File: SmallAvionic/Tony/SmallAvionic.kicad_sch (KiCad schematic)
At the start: 0 parts

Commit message: 完成基本開機電路
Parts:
- added C1, C2, C3, C4, C6, C9: 100n, symbol Device:C
- added C5, C7: 10u, symbol Device:C
- added C8: 1n, symbol Device:C
- added FB1: FerriteBead 120R @ 100M, symbol Device:FerriteBead
- added J1: Conn_01x02_Pin, symbol Connector:Conn_01x02_Pin
- added R1, R2: 10k, symbol Device:R
- added SW1: SW_Push, symbol Switch:SW_Push
- added TP1: TestPoint, symbol Connector:TestPoint
- added U1: STM32F103C8Tx, Package_QFP:LQFP-48_7x7mm_P0.5mm, symbol MCU_ST_STM32F1:STM32F103C8Tx
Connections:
- new net: C8.1, FB1.2
- new net: C9.1, SW1.2, U1.7 (NRST)
- new net: R1.1, TP1.1, U1.44 (BOOT0)
- new net: R2.1, U1.20 (PB2)
- new net +3.3V: C1.1, C2.1, C3.1, C4.1, C5.1, U1.1 (VBAT), U1.24 (VDD), U1.36 (VDD), U1.48 (VDD)
- new net +3.3VA: C6.1, C7.1, FB1.1, U1.9 (VDDA)
- new net GND: C1.2, C2.2, C3.2, C4.2, C5.2, C6.2, C7.2, C8.2, C9.2, R1.2, R2.2, SW1.1, U1.23 (VSS), U1.35 (VSS), U1.47 (VSS), U1.8 (VSSA)

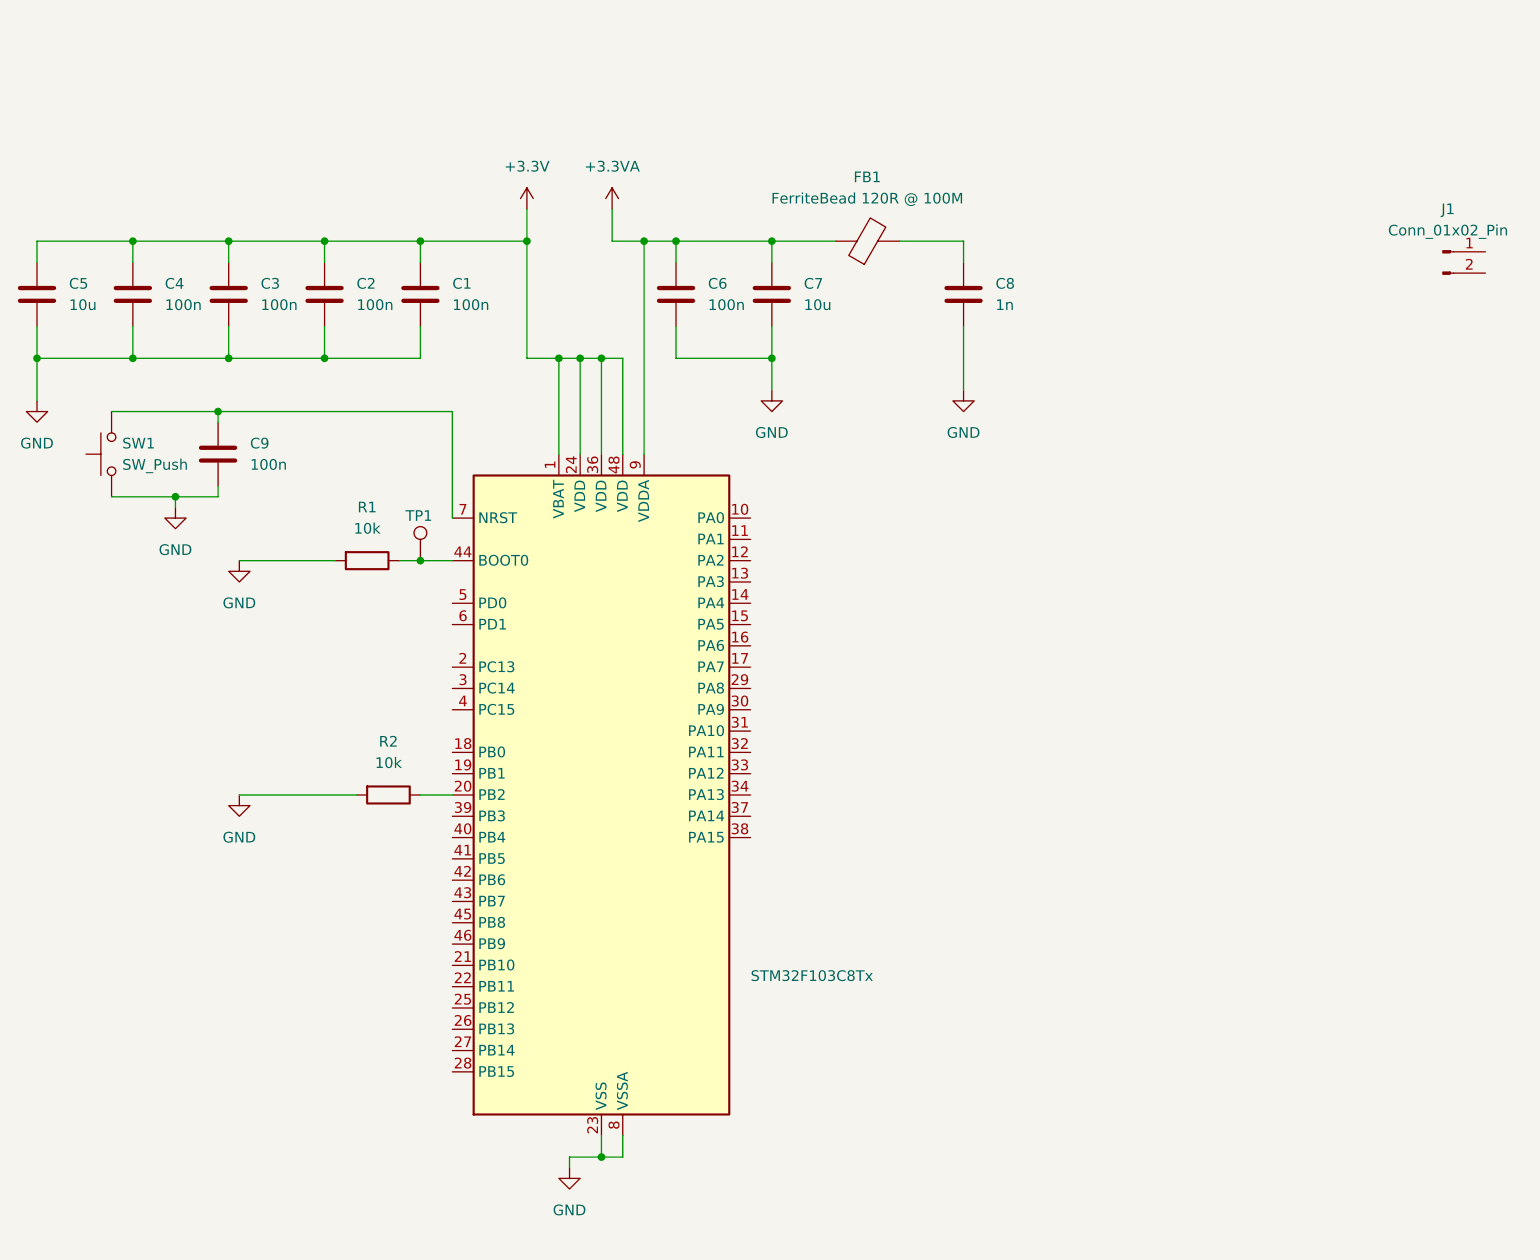
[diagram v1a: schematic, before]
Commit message: 進度到usb
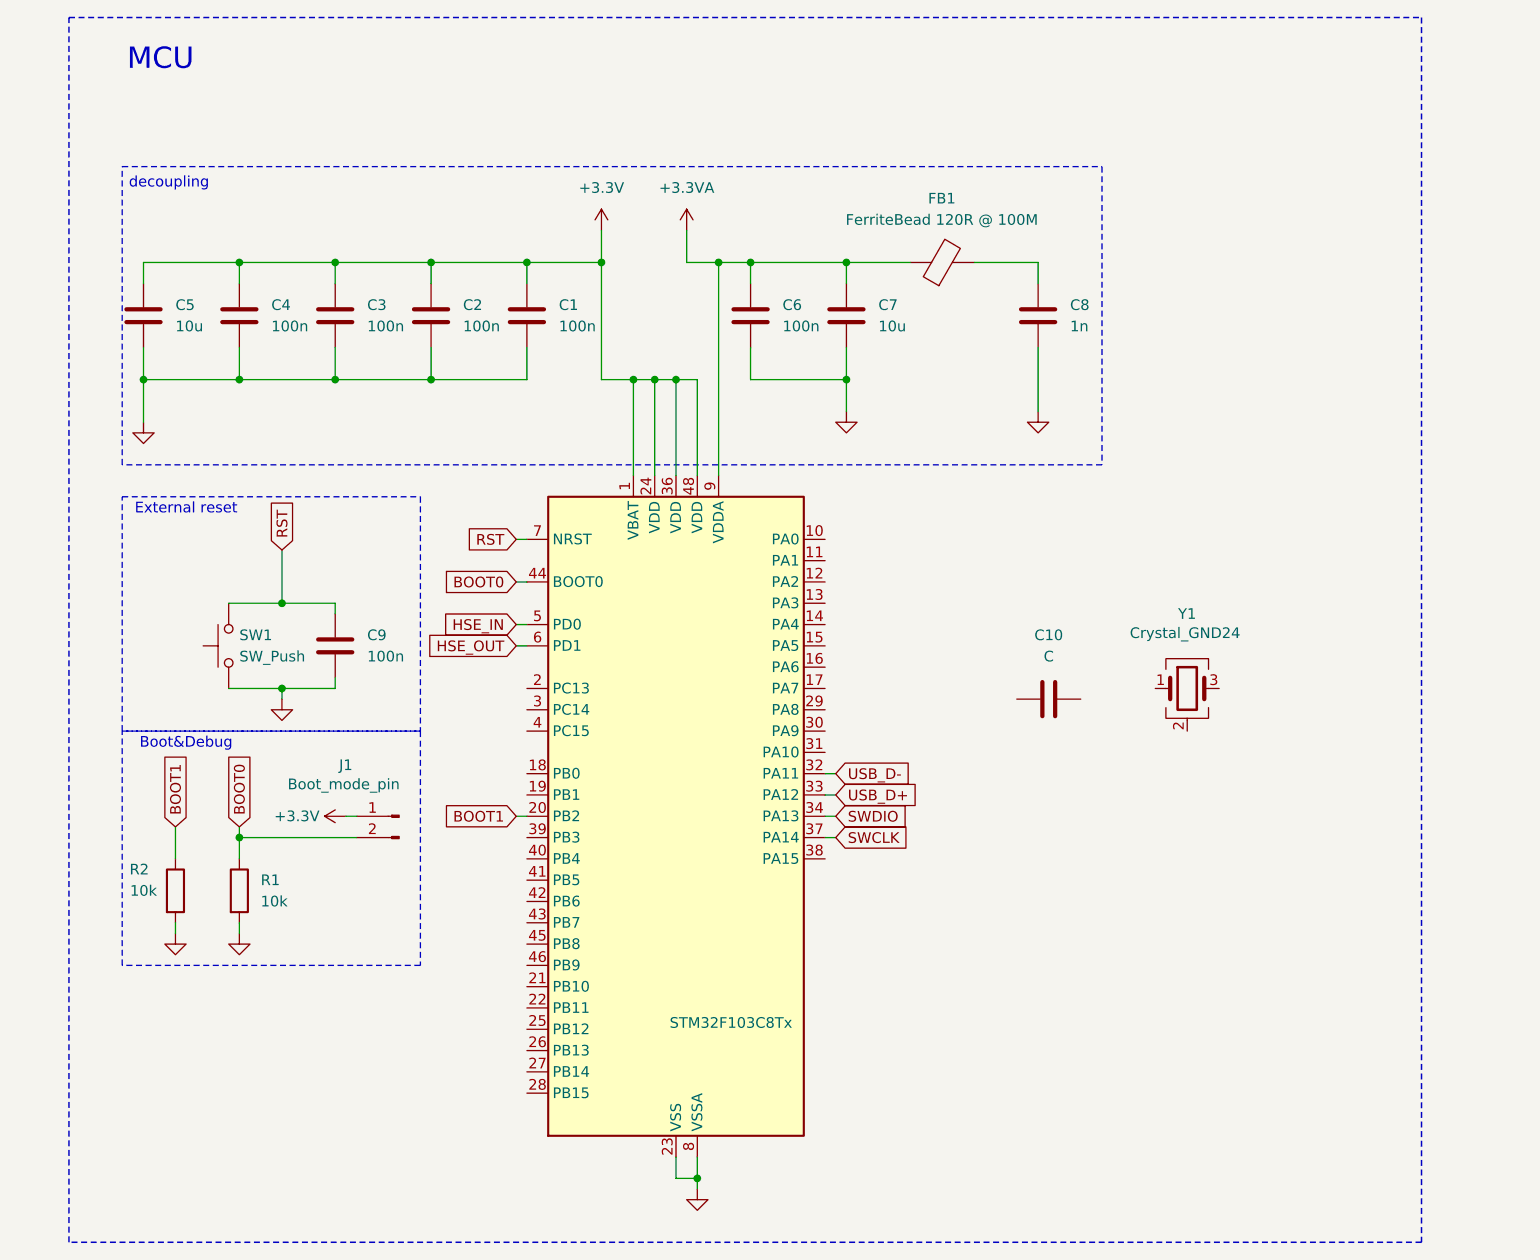
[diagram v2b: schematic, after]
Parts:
- removed TP1: TestPoint, symbol Connector:TestPoint
- added C10: C, symbol Device:C
- added Y1: Crystal_GND24, symbol Device:Crystal_GND24
- J1: value Conn_01x02_Pin -> Boot_mode_pin
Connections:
- net +3.3V: now also J1.1 (Pin_1)
- net RST: now reaches C9.1, SW1.2, U1.7 (NRST)
- net BOOT0: now reaches R1.1, U1.44 (BOOT0)
- net BOOT0: now also J1.2 (Pin_2)
- net BOOT1: now reaches R2.1, U1.20 (PB2)
- net USB_D-: now reaches U1.32 (PA11)
- net USB_D+: now reaches U1.33 (PA12)
- net SWDIO: now reaches U1.34 (PA13)
- net SWCLK: now reaches U1.37 (PA14)
- net HSE_IN: now reaches U1.5 (PD0)
- net HSE_OUT: now reaches U1.6 (PD1)
- new net: Y1.2 (G), Y1.4 (G)
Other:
- note added: "Boot&Debug"
- note added: "External reset"
- note added: "MCU"
- note added: "decoupling"
- moved on the sheet: C1, C2, C3, C4, C5, C6, C7, C8, C9, FB1, J1, R1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

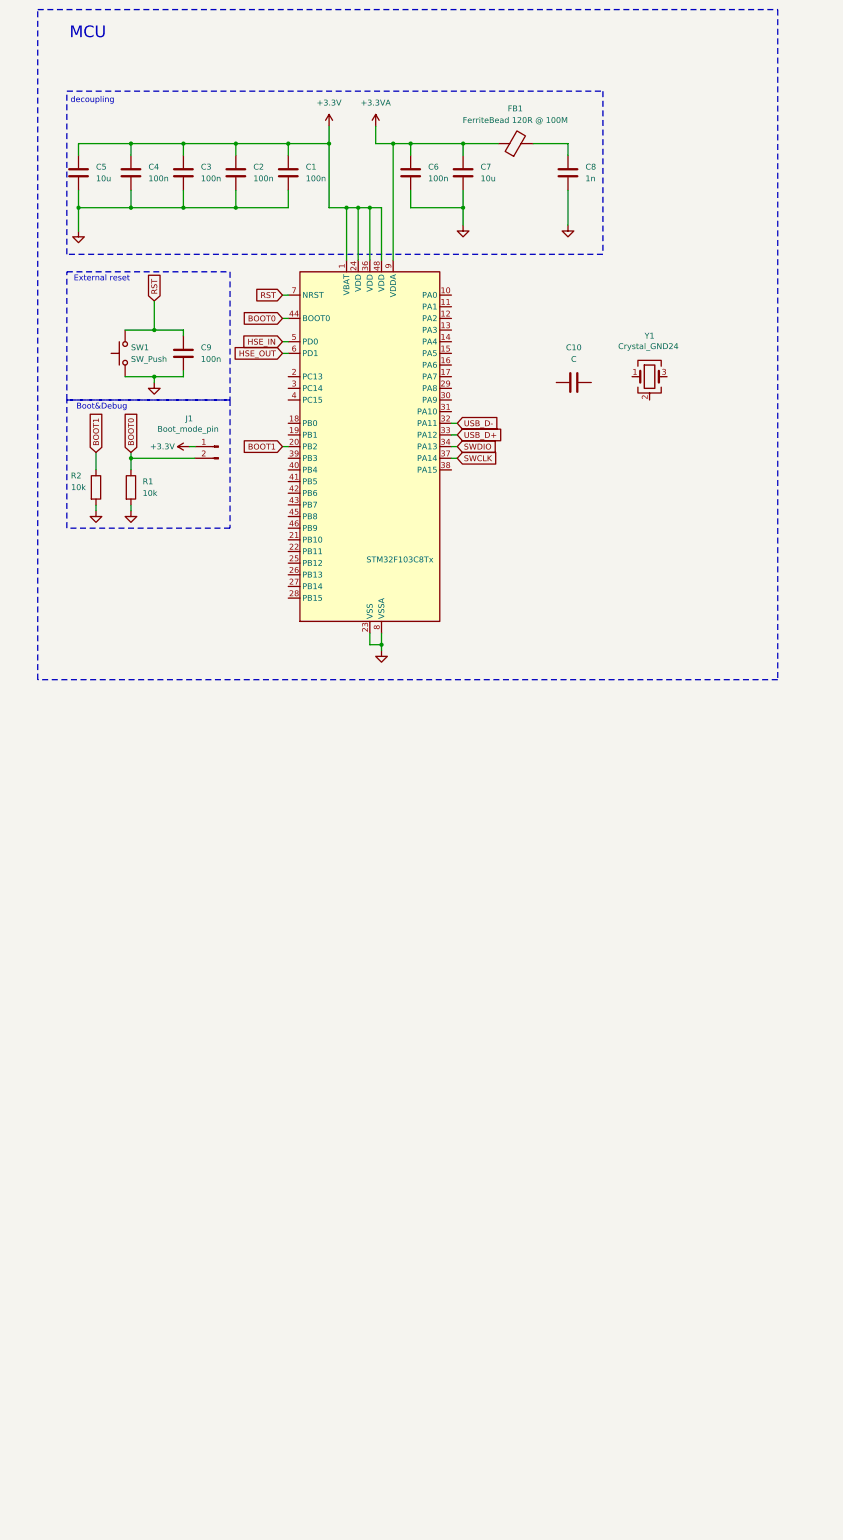
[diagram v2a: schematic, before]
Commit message: 1-25
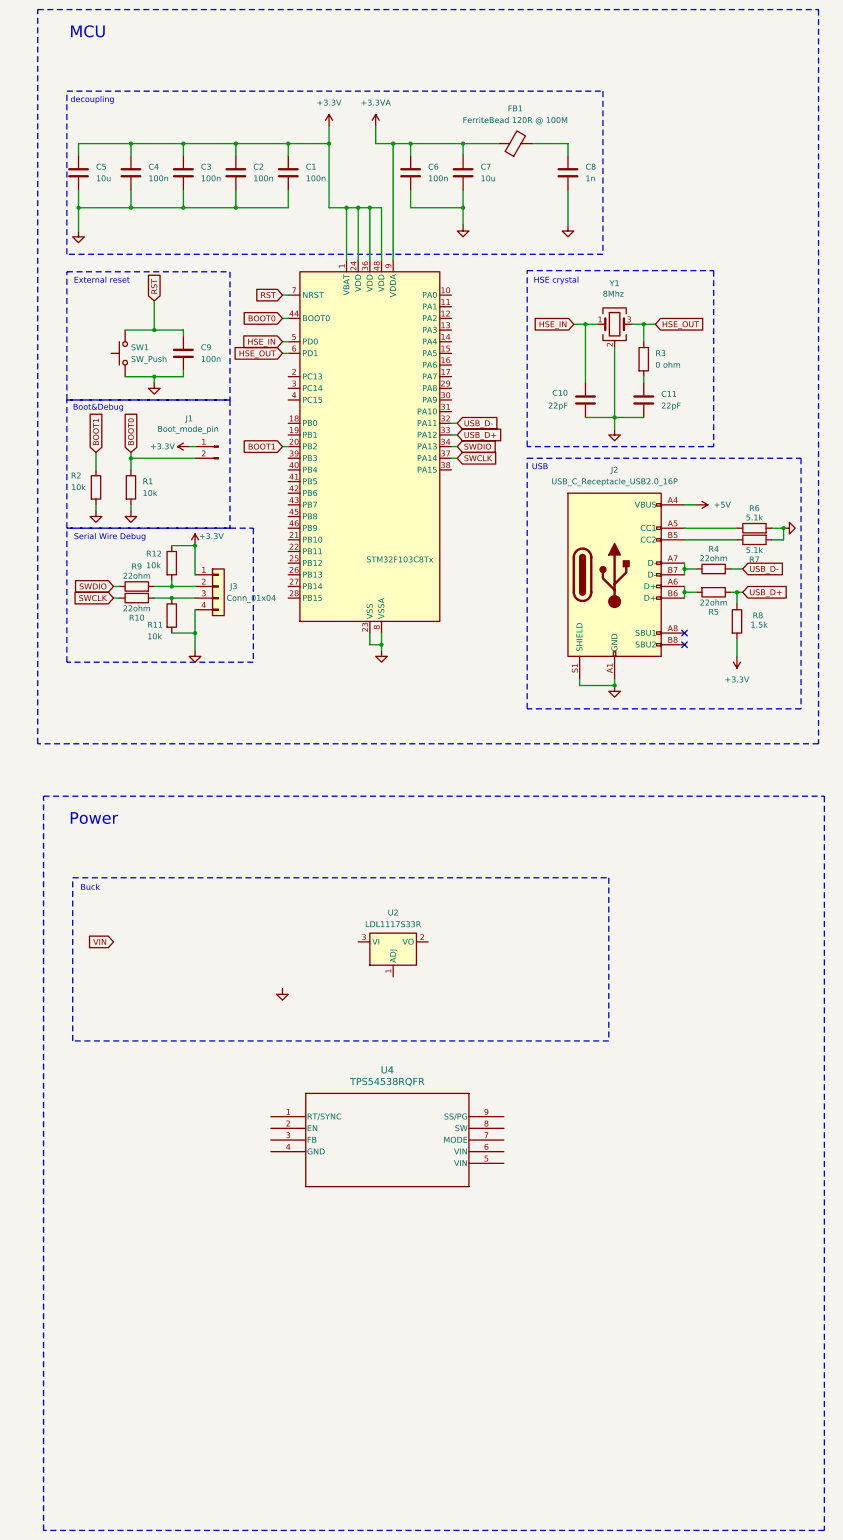
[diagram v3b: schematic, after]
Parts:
- added C11: 22pF, symbol Device:C
- added J2: USB_C_Receptacle_USB2.0_16P, symbol Connector:USB_C_Receptacle_USB2.0_16P
- added J3: Conn_01x04, symbol Connector_Generic:Conn_01x04
- added R10, R4, R5, R9: 22ohm, symbol Device:R
- added R11, R12: 10k, symbol Device:R
- added R3: 0 ohm, symbol Device:R
- added R6, R7: 5.1k, symbol Device:R
- added R8: 1.5k, symbol Device:R
- added U2: LDL1117S33R, Package_TO_SOT_SMD:SOT-223-3_TabPin2, symbol Regulator_Linear:AMS1117
- added U4: TPS54538RQFR, VQFN-HR9_RQF_TEX, symbol Small_av_tony_lib:TPS54538RQFR
- C10: value C -> 22pF
- Y1: value Crystal_GND24 -> 8Mhz
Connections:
- net +3.3V: now also J3.1 (Pin_1), R12.1, R8.2
- net GND: now also C10.2, Y1.2 (G), Y1.4 (G), C11.2, J2.A1 (GND), J2.A12 (GND), J2.B1 (GND), J2.B12 (GND), J2.S1 (SHIELD), J3.4 (Pin_4), R11.2, R6.2, R7.2
- net HSE_IN: now also C10.1, Y1.1
- net HSE_OUT: now also Y1.3, R3.1
- net SWCLK: now also R10.1
- net SWDIO: now also R9.1
- net USB_D+: now also R5.1, R8.1
- net USB_D-: now also R4.2
- new net: J2.A7 (D-), J2.B7 (D-), R4.1
- new net: J2.A5 (CC1), R6.1
- new net: J2.A6 (D+), J2.B6 (D+), R5.2
- new net: J2.B5 (CC2), R7.1
- new net: C11.1, R3.2
- new net: J3.3 (Pin_3), R10.2, R11.1
- new net: J3.2 (Pin_2), R12.2, R9.2
- new net +5V: J2.A4 (VBUS), J2.A9 (VBUS), J2.B4 (VBUS), J2.B9 (VBUS)
- no-connect marks 0 -> 2
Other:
- note added: "Buck"
- note added: "HSE crystal"
- note added: "Power"
- note added: "Serial Wire Debug"
- note added: "USB"
- moved on the sheet: Y1
